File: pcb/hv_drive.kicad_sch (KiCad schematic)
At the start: 47 parts, among them Q1 IGD70R500, Q2 PNP, Q3 NPN, U5 DA2032-AL, U6 UA7810, U7 TL431DBZ, U8 PC817, U9 UC3842_SOIC14

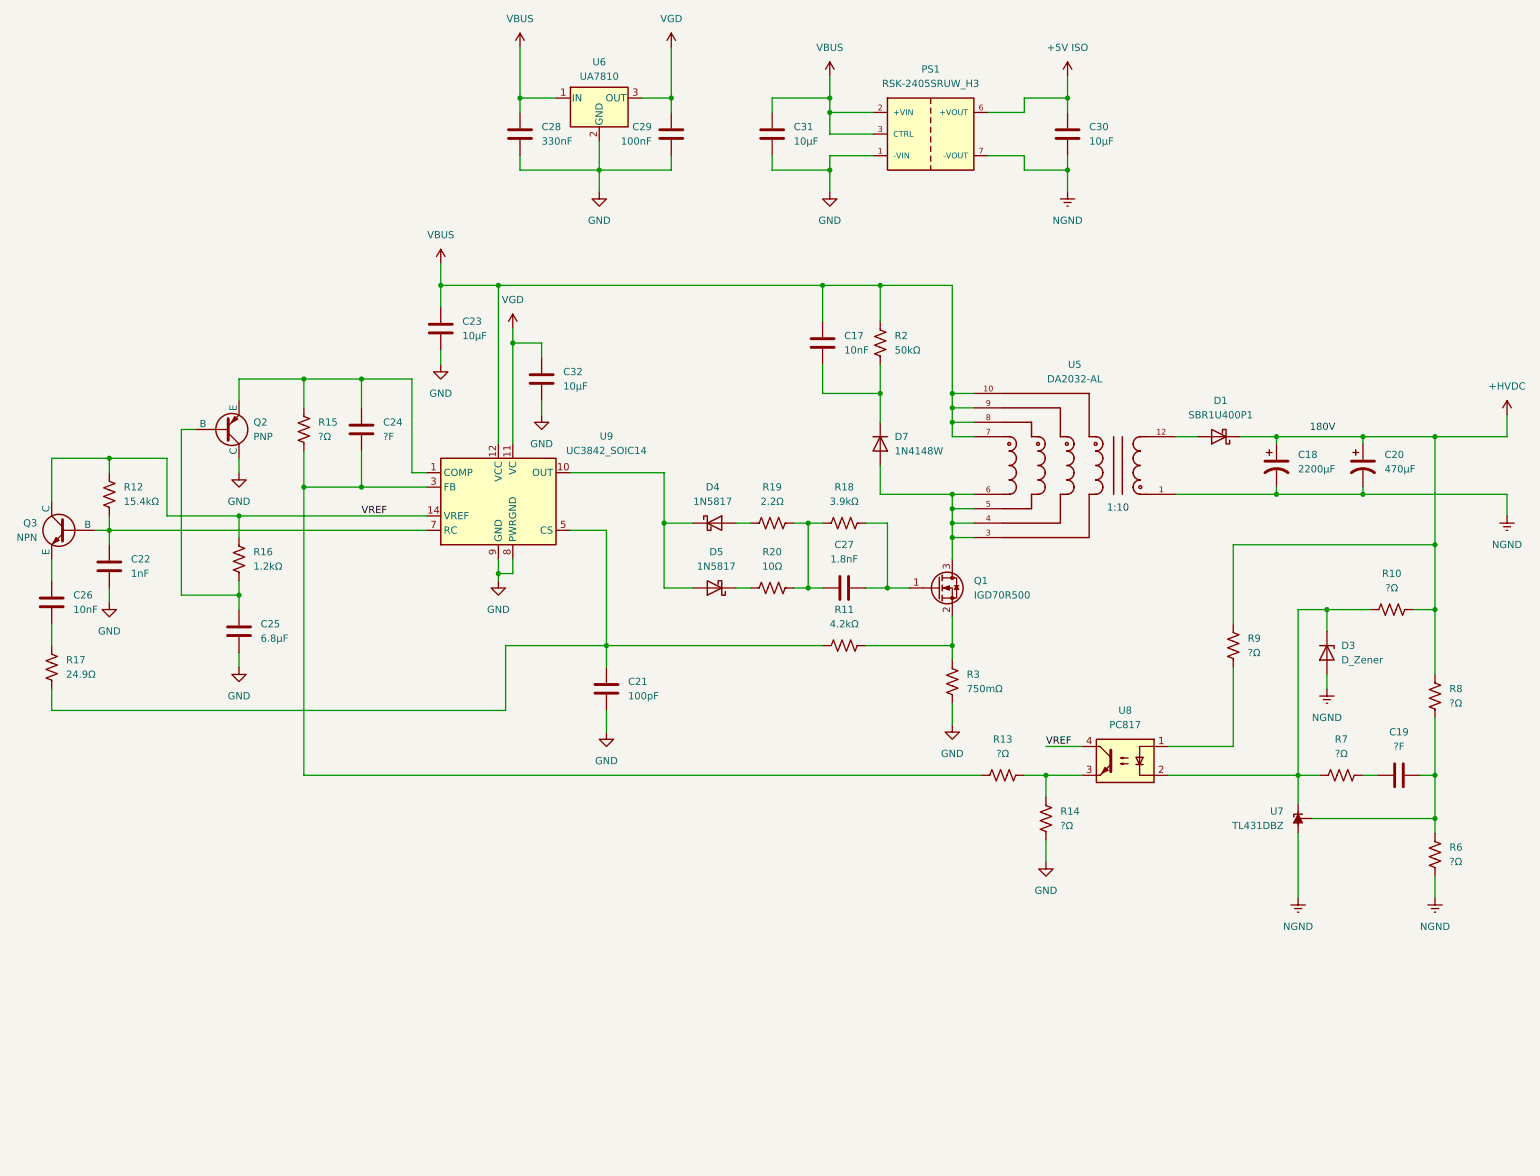
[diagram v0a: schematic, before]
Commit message: w
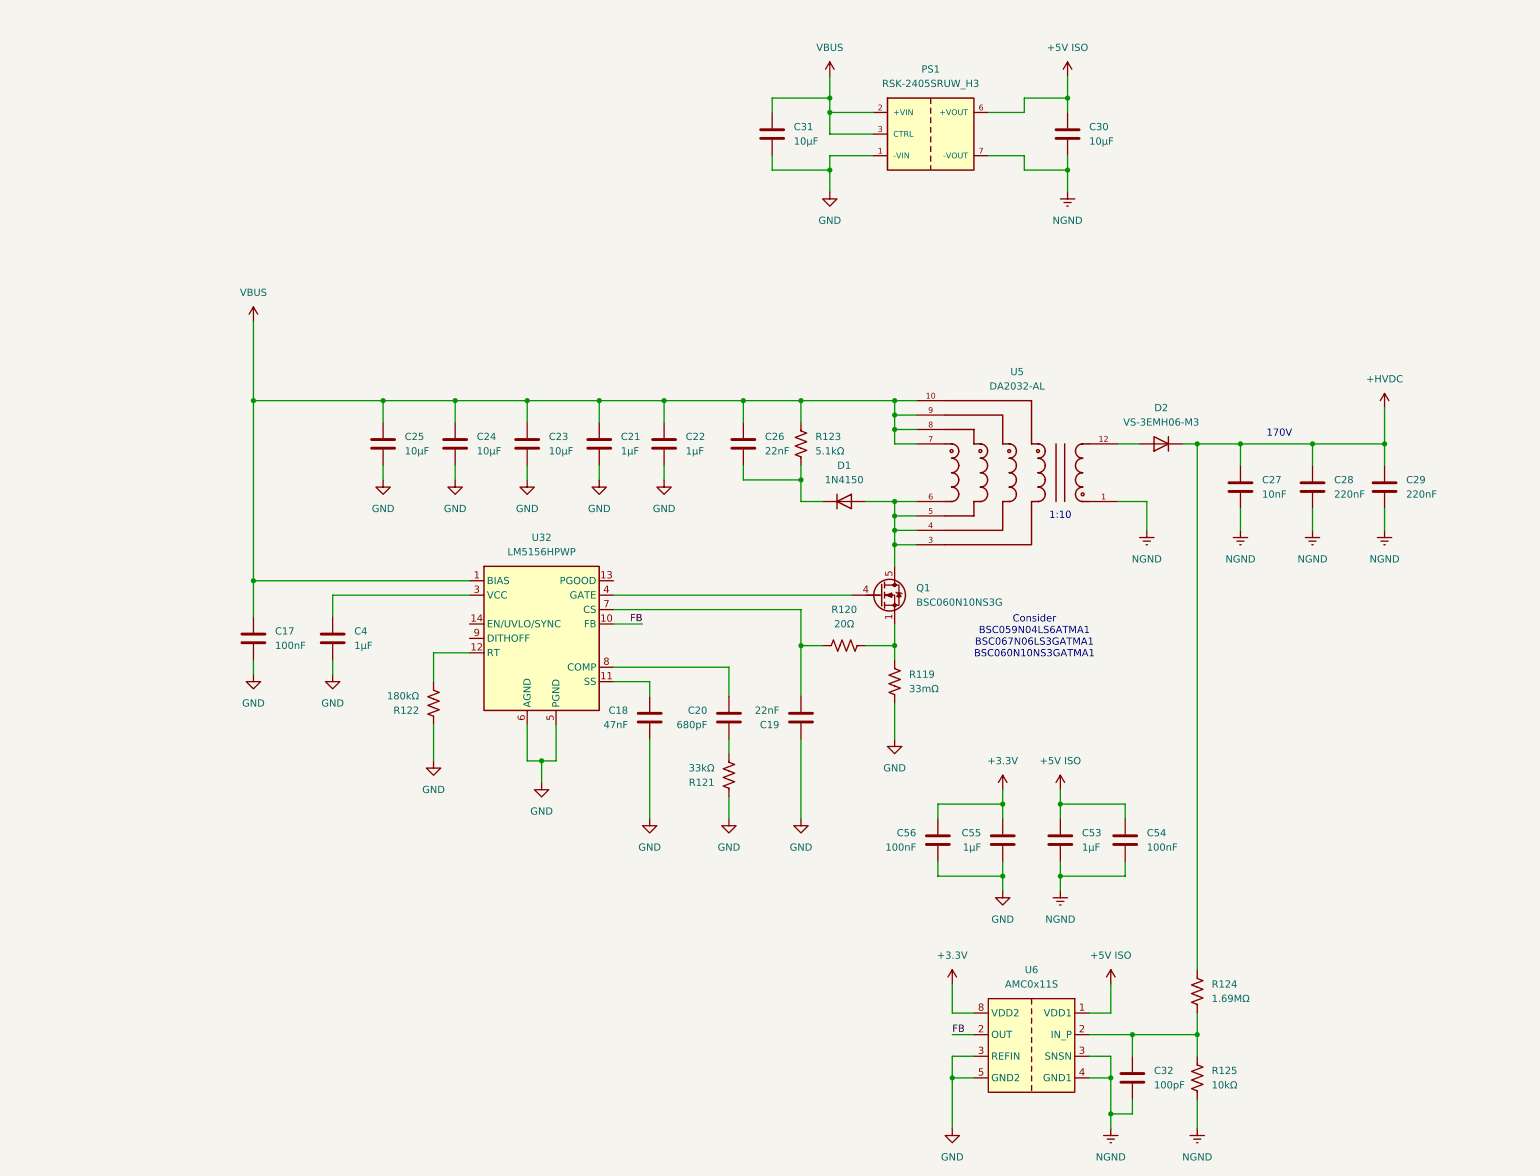
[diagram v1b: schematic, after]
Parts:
- removed C18: 2200μF, Capacitor_SMD:C_1206_3216Metric_Pad1.33x1.80mm_HandSolder, symbol Device:C_Polarized_US
- removed C20: 470μF, Capacitor_SMD:C_1206_3216Metric_Pad1.33x1.80mm_HandSolder, symbol Device:C_Polarized_US
- removed D1: SBR1U400P1, symbol Device:D_Schottky
- removed D3: D_Zener, symbol Device:D_Zener
- removed D4, D5: 1N5817, Diode_THT:D_DO-41_SOD81_P10.16mm_Horizontal, symbol Diode:1N5817
- removed D7: 1N4148W, Diode_SMD:D_SOD-123, symbol Diode:1N4148W
- removed Q1: IGD70R500, Package_TO_SOT_SMD:TO-252-2, symbol Transistor_FET:Q_NMOS_GSD
- removed Q2: PNP, symbol Simulation_SPICE:PNP
- removed Q3: NPN, symbol Simulation_SPICE:NPN
- removed R10, R13, R14, R15, R6, R7, R8, R9: ?Ω, Resistor_SMD:R_1206_3216Metric_Pad1.30x1.75mm_HandSolder, symbol Device:R_US
- removed R11: 4.2kΩ, Resistor_SMD:R_1206_3216Metric_Pad1.30x1.75mm_HandSolder, symbol Device:R_US
- removed R12: 15.4kΩ, Resistor_SMD:R_1206_3216Metric_Pad1.30x1.75mm_HandSolder, symbol Device:R_US
- removed R16: 1.2kΩ, Resistor_SMD:R_1206_3216Metric_Pad1.30x1.75mm_HandSolder, symbol Device:R_US
- removed R17: 24.9Ω, Resistor_SMD:R_1206_3216Metric_Pad1.30x1.75mm_HandSolder, symbol Device:R_US
- removed R18: 3.9kΩ, Resistor_SMD:R_1206_3216Metric_Pad1.30x1.75mm_HandSolder, symbol Device:R_US
- removed R19: 2.2Ω, Resistor_SMD:R_1206_3216Metric_Pad1.30x1.75mm_HandSolder, symbol Device:R_US
- removed R2: 50kΩ, Resistor_SMD:R_1206_3216Metric_Pad1.30x1.75mm_HandSolder, symbol Device:R_US
- removed R20: 10Ω, Resistor_SMD:R_1206_3216Metric_Pad1.30x1.75mm_HandSolder, symbol Device:R_US
- removed R3: 750mΩ, Resistor_SMD:R_1206_3216Metric_Pad1.30x1.75mm_HandSolder, symbol Device:R_US
- removed U6: UA7810, Package_TO_SOT_THT:TO-220-3_Vertical, symbol Regulator_Linear:uA7810
- removed U7: TL431DBZ, Package_TO_SOT_SMD:SOT-23, symbol Reference_Voltage:TL431DBZ
- removed U8: PC817, Package_DIP:DIP-4_W7.62mm, symbol Isolator:PC817
- removed U9: UC3842_SOIC14, Package_SO:SOIC-14_3.9x8.7mm_P1.27mm, symbol Regulator_Controller:UC3842_SOIC14
- added C18: 47nF, Capacitor_SMD:C_1206_3216Metric_Pad1.33x1.80mm_HandSolder, symbol Device:C
- added C20: 680pF, Capacitor_SMD:C_1206_3216Metric_Pad1.33x1.80mm_HandSolder, symbol Device:C
- added C4, C53, C55: 1μF, Capacitor_SMD:C_1206_3216Metric_Pad1.33x1.80mm_HandSolder, symbol Device:C
- added C54, C56: 100nF, Capacitor_SMD:C_1206_3216Metric_Pad1.33x1.80mm_HandSolder, symbol Device:C
- added D1: 1N4150, Diode_SMD:Nexperia_CFP3_SOD-123W, symbol Device:D
- added D2: VS-3EMH06-M3, Diode_SMD:D_SMA_Handsoldering, symbol Device:D
- added Q1: BSC060N10NS3G, Package_TO_SOT_SMD:TDSON-8-1, symbol Transistor_FET:BSC060N10NS3G
- added R119: 33mΩ, Resistor_SMD:R_1206_3216Metric_Pad1.30x1.75mm_HandSolder, symbol Device:R_US
- added R120: 20Ω, Resistor_SMD:R_1206_3216Metric_Pad1.30x1.75mm_HandSolder, symbol Device:R_US
- added R121: 33kΩ, Resistor_SMD:R_1206_3216Metric_Pad1.30x1.75mm_HandSolder, symbol Device:R_US
- added R122: 180kΩ, Resistor_SMD:R_1206_3216Metric_Pad1.30x1.75mm_HandSolder, symbol Device:R_US
- added R123: 5.1kΩ, Resistor_SMD:R_1206_3216Metric_Pad1.30x1.75mm_HandSolder, symbol Device:R_US
- added R124: 1.69MΩ, Resistor_SMD:R_1206_3216Metric_Pad1.30x1.75mm_HandSolder, symbol Device:R_US
- added R125: 10kΩ, Resistor_SMD:R_1206_3216Metric_Pad1.30x1.75mm_HandSolder, symbol Device:R_US
- added U32: LM5156HPWP, Package_SO:Texas_HTSSOP-14-1EP_4.4x5mm_P0.65mm_EP3.4x5mm_Mask3.155x3.255mm_ThermalVias, symbol Regulator_Switching:LM5156HPWP
- added U6: AMC0x11S, symbol Symbols:AMC0x11S
- C17: value 10nF -> 100nF; Manufacturer Part Number (none) -> C1206C104K5RACTU; Vendor Part Number (none) -> 399-C1206C104K5RACTUCT-ND
- C19: value ?F -> 22nF; Manufacturer Part Number (none) -> C1206C104K5RACTU; Vendor Part Number (none) -> 399-C1206C104K5RACTUCT-ND
- C21: value 100pF -> 1μF; Manufacturer Part Number (none) -> CL31B105KAHNNNE; Vendor Part Number (none) -> 1276-1097-1-ND
- C22: value 1nF -> 1μF; Manufacturer Part Number (none) -> CL31B105KAHNNNE; Vendor Part Number (none) -> 1276-1097-1-ND
- C23: Manufacturer Part Number CL31A106MAHNNNE -> CL31B105KAHNNNE; Vendor Part Number 1276-1181-1-ND -> 1276-1097-1-ND
- C24: value ?F -> 10μF; Manufacturer Part Number (none) -> CL31B105KAHNNNE; Vendor Part Number (none) -> 1276-1097-1-ND
- C25: value 6.8μF -> 10μF; Manufacturer Part Number (none) -> CL31B105KAHNNNE; Vendor Part Number (none) -> 1276-1097-1-ND
- C26: value 10nF -> 22nF; Manufacturer Part Number (none) -> C1206C104K5RACTU; Vendor Part Number (none) -> 399-C1206C104K5RACTUCT-ND
- C27: value 1.8nF -> 10nF; Manufacturer Part Number (none) -> C1206C104K5RACTU; Vendor Part Number (none) -> 399-C1206C104K5RACTUCT-ND
- C28: value 330nF -> 220nF; Manufacturer Part Number (none) -> C1206C104K5RACTU; Vendor Part Number (none) -> 399-C1206C104K5RACTUCT-ND
- C29: value 100nF -> 220nF
- C32: value 10μF -> 100pF; Manufacturer Part Number CL31A106MAHNNNE -> (none); Vendor Part Number 1276-1181-1-ND -> (none)
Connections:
- net +5V ISO: now also C53.1, C54.1, U6.1 (VDD1)
- net +HVDC: now also C27.1, C28.1, C29.1, D2.1 (K), R124.2
- net GND: now also C17.2, C19.1, C22.2, C24.2, C25.2, C18.2, C4.2, C55.2, C56.2, R119.2, R121.1, R122.1, U32.15 (AGND), U32.5 (PGND), U32.6 (AGND), U6.3 (REFIN), U6.5 (GND2); no longer C22.1, C25.1, C28.2, C29.2, C32.2
- net NGND: now also C27.2, C28.2, C29.2, C32.1, C53.2, C54.2, R125.1, U6.3 (REFIN), U6.4 (GND1)
- net VBUS: now also C21.1, C22.1, C24.1, C25.1, C26.1, R123.1, U32.1 (BIAS); no longer C28.1
- net at U5.12: now also D2.2 (A)
- net at U5.3, U5.4, U5.5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: now also D1.2 (A), Q1.5 (D)
- net at C19.2: now also R120.1, U32.7 (CS)
- net at C26.2: now also D1.1 (K), R123.2
- removed net VGD: C29.1, C32.1
- new net: C18.1, U32.11 (SS)
- new net: Q1.1 (S), Q1.2 (S), Q1.3 (S), R119.1, R120.2
- new net: C32.2, R124.1, R125.2, U6.2 (OUT)
- new net: C20.2, R121.2
- new net: R122.2, U32.12 (RT)
- new net: C4.1, U32.3 (VCC)
- new net: Q1.4 (G), U32.4 (GATE)
- new net: C20.1, U32.8 (COMP)
- new net +3.3V: C55.1, C56.1, U6.8 (VDD2)
- new net FB: U32.10 (FB), U6.2 (OUT)
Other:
- note added: "170V"
- note added: "Consider BSC059N04LS6ATMA1 BSC067N06LS3GATMA1 BSC060N10NS3GATMA1"
- note removed: "180V"
- moved on the sheet: U5
